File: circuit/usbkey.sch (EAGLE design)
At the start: 29 parts, among them IC1 ATmega168P, Q1 16MHz, X1 1503_09, X2 USB

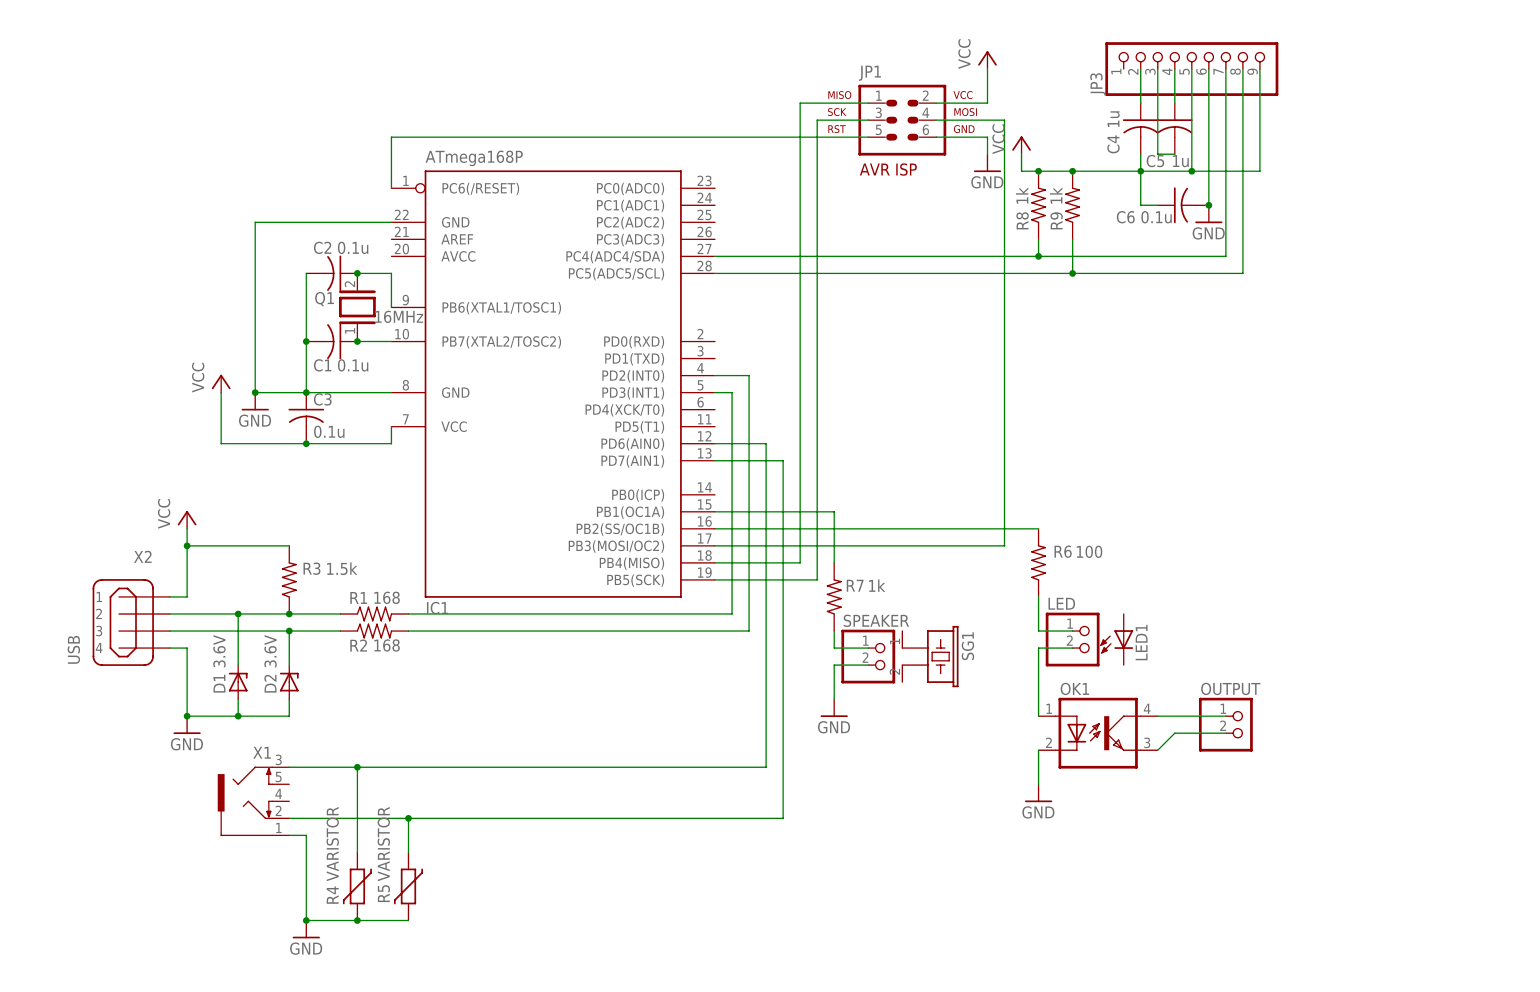
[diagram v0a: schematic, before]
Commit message: update
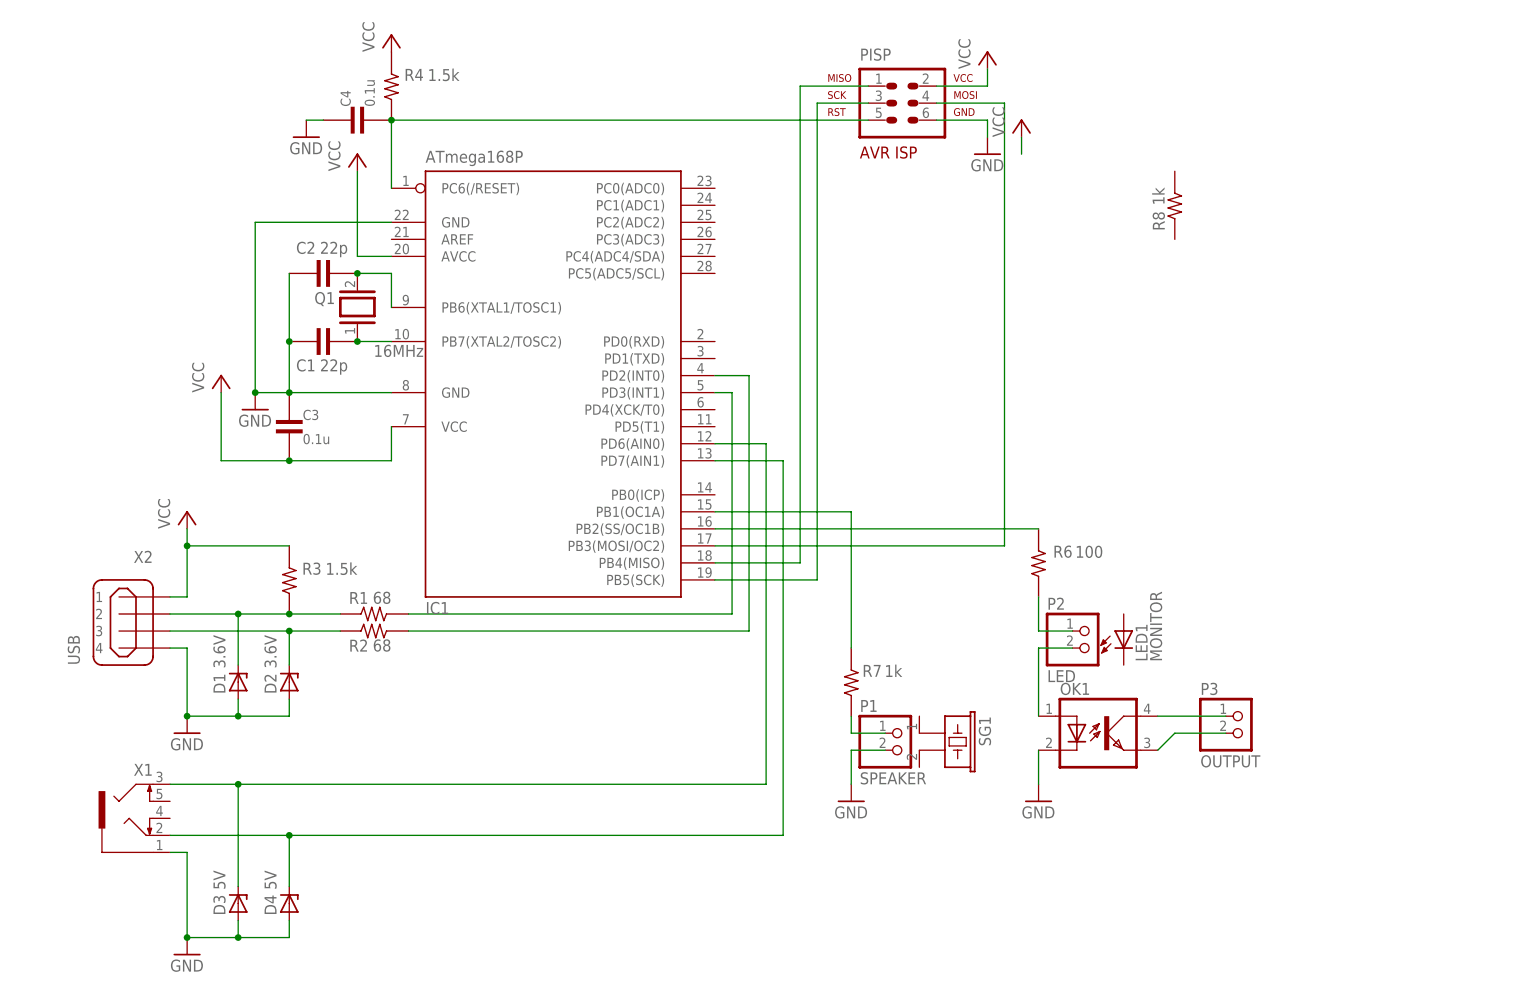
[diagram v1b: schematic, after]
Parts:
- removed C5: 1u, resistor:C-US025-024X044
- removed C6: 0.1u, resistor:C-US025-024X044
- removed JP1: AVR-ISP-6VERT, avr-7:AVR-ISP-6VERT
- removed JP3: (no value), pinhead:PINHD-1X9
- removed R5: VARISTOR, varistor:VARISTOR-2,5
- removed R9: 1k, resistor:R-US_0204/7
- removed SPEAKER: (no value), pinhead:PINHD-1X2
- added D3, D4: 5V, diode:BZX55
- added P1: SPEAKER, pinhead:PINHD-1X2
- added PISP: AVR-ISP-6VERT, avr-7:AVR-ISP-6VERT
- C1, C2: value 0.1u -> 22p; device resistor:C-US025-024X044 -> c-j:C-50V-0302-2.54
- C3: device resistor:C-US025-024X044 -> c-j:C-50V-0302-2.54
- C4: value 1u -> 0.1u; device resistor:C-US025-024X044 -> c-j:C-50V-0302-2.54
- LED1: value (none) -> MONITOR
- P2: value (none) -> LED
- P3: value (none) -> OUTPUT
- R1, R2: value 168 -> 68; device resistor:R-US_0204/2V -> r-j:R-1/4W-07.62
- R3: device resistor:R-US_0204/7 -> r-j:R-1/4W-02.54-V
- R4: value VARISTOR -> 1.5k; device varistor:VARISTOR-2,5 -> r-j:R-1/4W-02.54-V
- R6: device resistor:R-US_0204/2V -> r-j:R-1/4W-02.54-V
- R7: device resistor:R-US_0204/2V -> r-j:R-1/4W-07.62
- R8: device resistor:R-US_0204/7 -> r-j:R-1/4W-07.62
- renumbered LED to P2, OUTPUT to P3
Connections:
- removed net N$20: C4.1, JP3.2
- removed net N$21: C5.1, JP3.4
- removed net N$22: C5.2, JP3.3
- removed net N$23: IC1.PC4(ADC4/SDA), JP3.7, R8.1
- removed net N$24: IC1.PC5(ADC5/SCL), JP3.8, R9.1
- net GND: now also C4.1, D3.A, D4.A, P1.2, PISP.6; no longer C6.2, JP1.6, JP3.6, R4.2, R5.2, SPEAKER.2
- net N$10: now also PISP.4; no longer JP1.4
- net N$11: now also PISP.3; no longer JP1.3
- net N$12: now also PISP.1; no longer JP1.1
- net N$14: now also P1.1; no longer SPEAKER.1
- net N$7: now also D3.C; no longer R4.1
- net N$8: now also D4.C; no longer R5.1
- net N$9: now also C4.2, PISP.5, R4.1; no longer JP1.5
- net VCC: now also IC1.AVCC, PISP.2, R4.2; no longer C4.2, C6.1, JP1.2, JP3.5, JP3.9, R8.2, R9.2
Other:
- moved on the sheet: SG1, X1

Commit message: update
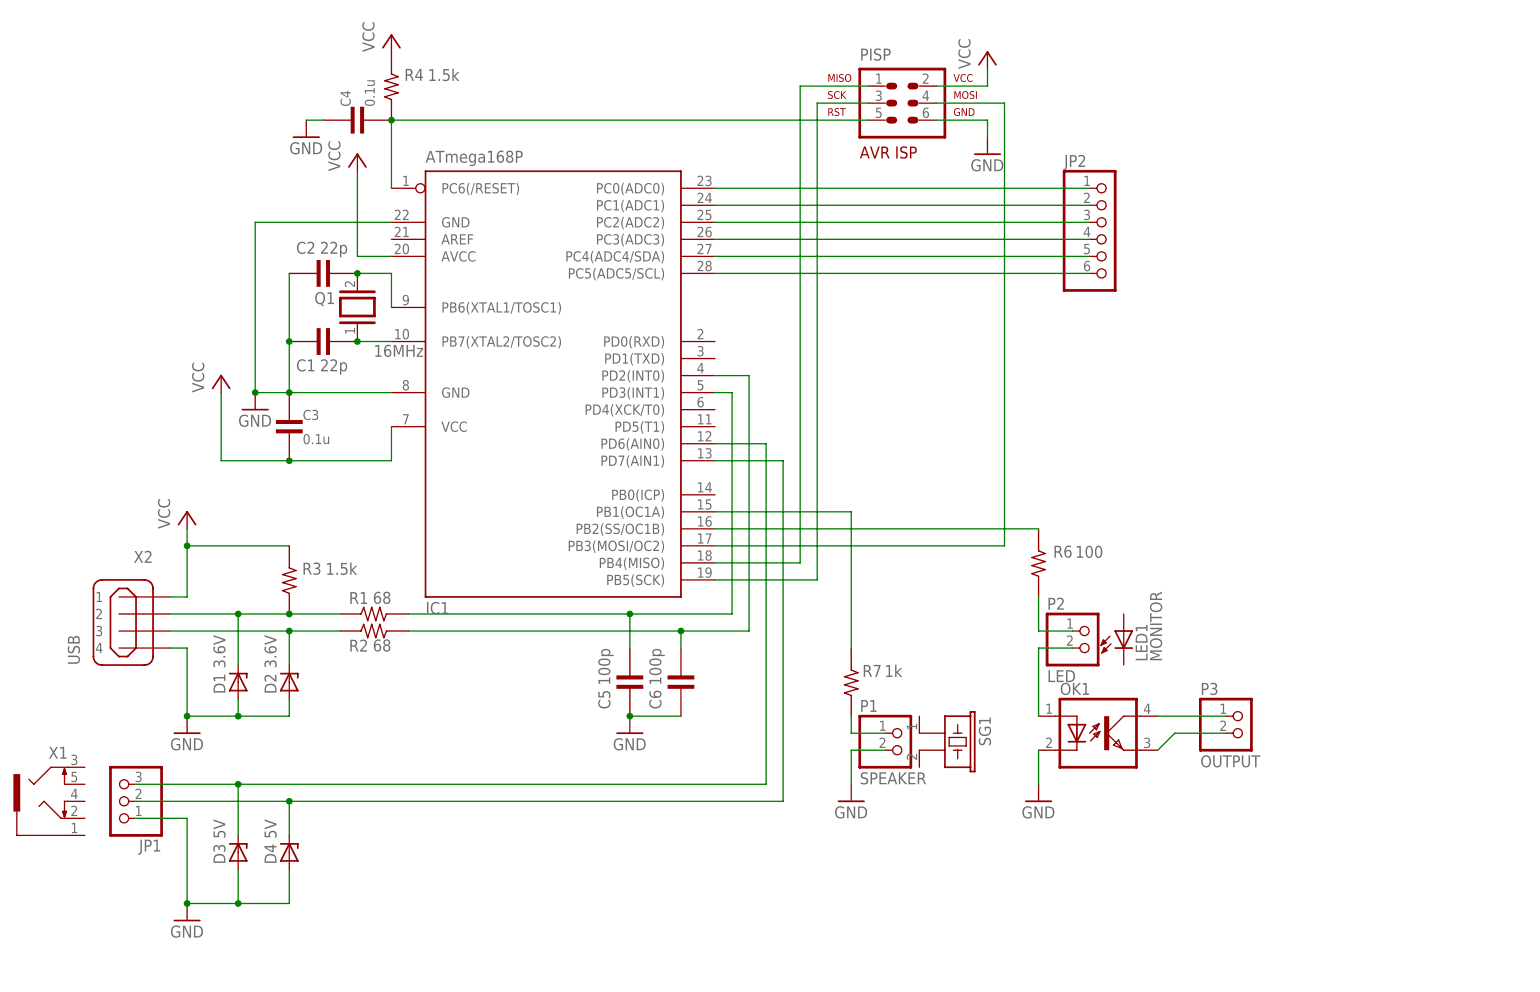
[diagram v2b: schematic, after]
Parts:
- removed R8: 1k, r-j:R-1/4W-07.62
- added C5, C6: 100p, c-j:C-50V-0302-2.54
- added JP1: (no value), pinhead:PINHD-1X3
- added JP2: (no value), pinhead:PINHD-1X6
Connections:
- new net N$20: IC1.PC0(ADC0), JP2.1
- new net N$21: IC1.PC1(ADC1), JP2.2
- new net N$22: IC1.PC2(ADC2), JP2.3
- new net N$23: IC1.PC3(ADC3), JP2.4
- new net N$24: IC1.PC4(ADC4/SDA), JP2.5
- new net N$25: IC1.PC5(ADC5/SCL), JP2.6
- net GND: now also C5.2, C6.2, JP1.1; no longer X1.1
- net N$3: now also C5.1
- net N$5: now also C6.1
- net N$7: now also JP1.3; no longer X1.3
- net N$8: now also JP1.2; no longer X1.2
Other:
- moved on the sheet: D3, D4, X1

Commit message: update
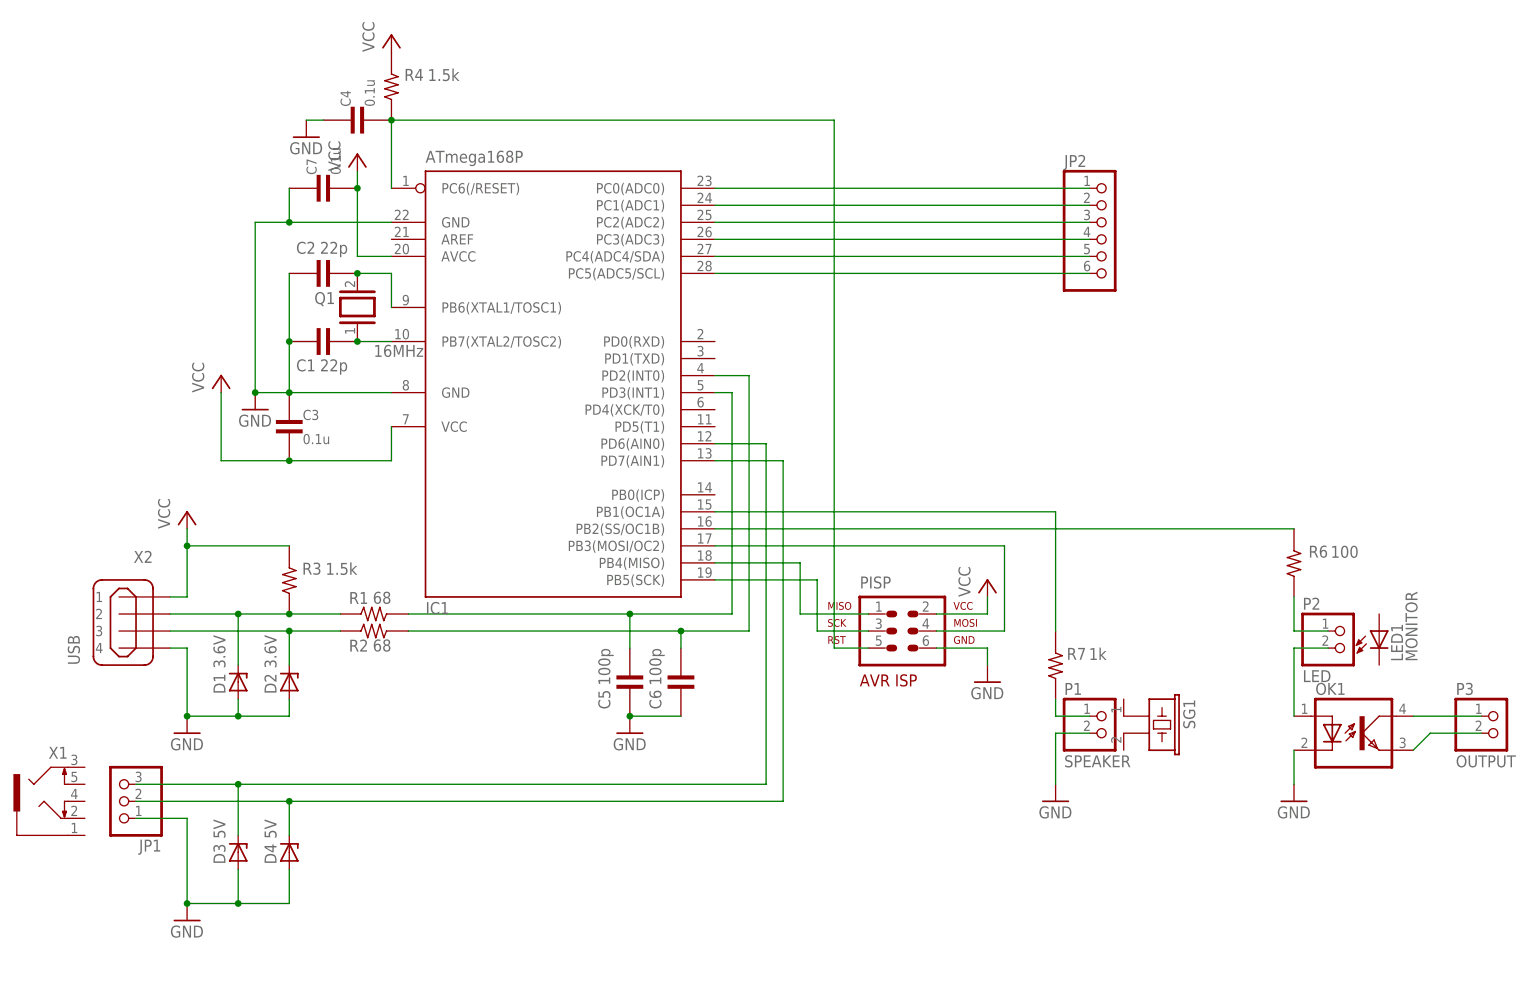
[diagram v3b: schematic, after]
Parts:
- added C7: 0.1u, c-j:C-50V-0302-2.54
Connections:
- net GND: now also C7.1
- net VCC: now also C7.2
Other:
- moved on the sheet: LED1, OK1, P1, P2, P3, PISP, R6, R7, SG1
